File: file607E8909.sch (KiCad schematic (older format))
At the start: 8 parts, among them J1 Conn_01x06_Female, U3 INA4180A1IPWR, U5 254

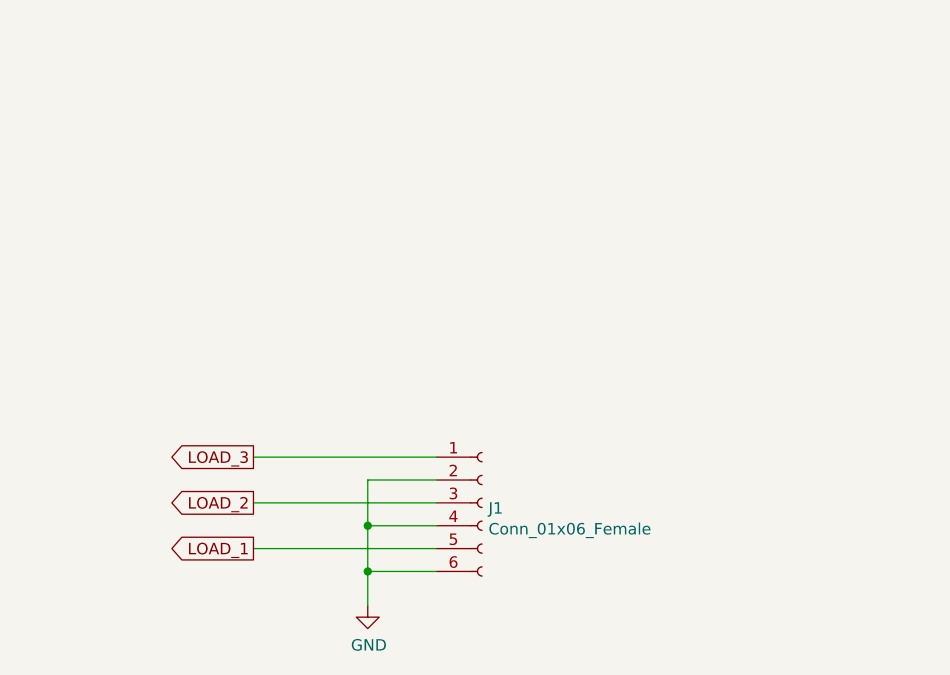
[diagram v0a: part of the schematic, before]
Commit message: incomplete pcb
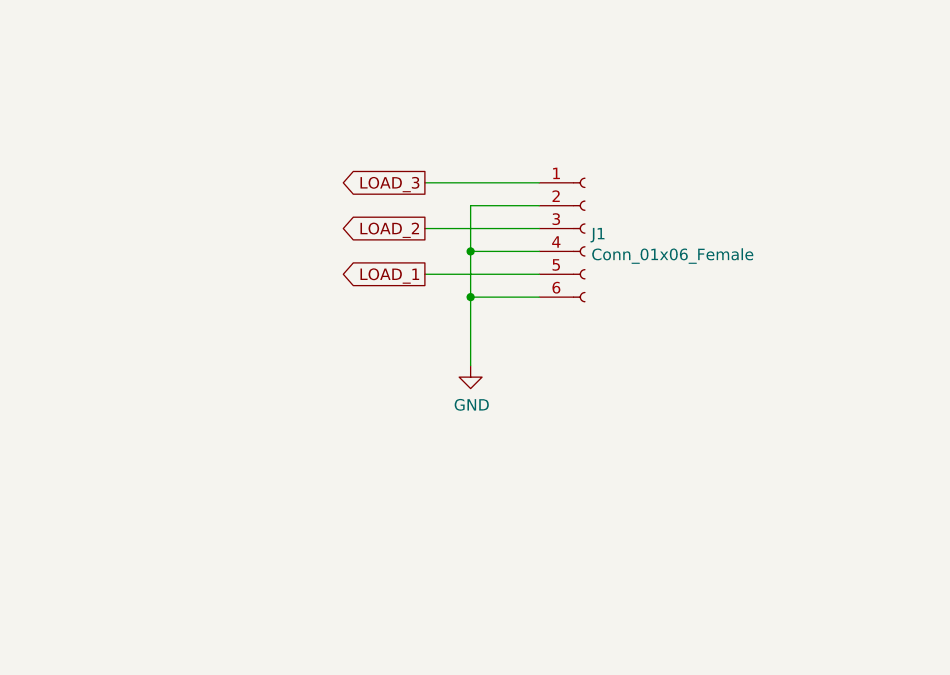
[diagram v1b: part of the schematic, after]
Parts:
- J1: footprint Connector_PinHeader_2.54mm:PinHeader_1x06_P2.54mm_Vertical -> Connector_PinSocket_2.54mm:PinSocket_1x06_P2.54mm_Vertical
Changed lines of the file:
@@
 	9950 2150 10150 2150
 NoConn ~ 10150 2150
+Text GLabel 2400 4150 0    50   Output ~ 0
+LOAD_3
+Wire Wire Line
+	2400 4150 2900 4150
+Wire Wire Line
+	2900 4250 2600 4250
+Wire Wire Line
+	2900 4450 2600 4450
+$Comp
+L power:GND #PWR066
+U 1 1 608EA451
+P 2600 4950
+F 0 "#PWR066" H 2600 4700 50  0001 C CNN
+F 1 "GND" H 2605 4777 50  0000 C CNN
+F 2 "" H 2600 4950 50  0001 C CNN
+F 3 "" H 2600 4950 50  0001 C CNN
+	1    2600 4950
+	1    0    0    -1
+$EndComp
+Text GLabel 2400 4350 0    50   Output ~ 0
+LOAD_2
+Text GLabel 2400 4550 0    50   Output ~ 0
+LOAD_1
+Wire Wire Line
+	2400 4550 2900 4550
 $Comp
 L Connector:Conn_01x06_Female J1
-U 1 1 608A75AE
-P 2650 5550
-F 0 "J1" H 2678 5526 50  0000 L CNN
-F 1 "Conn_01x06_Female" H 2678 5435 50  0000 L CNN
-F 2 "Connector_PinHeader_2.54mm:PinHeader_1x06_P2.54mm_Vertical" H 2650 5550 50  0001 C CNN
-F 3 "~" H 2650 5550 50  0001 C CNN
-	1    2650 5550
-	1    0    0    -1
-$EndComp
-$Comp
-L power:GND #PWR029
-U 1 1 608A8BC9
-P 2150 6000
-F 0 "#PWR029" H 2150 5750 50  0001 C CNN
-F 1 "GND" H 2155 5827 50  0000 C CNN
-F 2 "" H 2150 6000 50  0001 C CNN
-F 3 "" H 2150 6000 50  0001 C CNN
-	1    2150 6000
+U 1 1 6091EFB8
+P 3100 4350
+F 0 "J1" H 3128 4326 50  0000 L CNN
+F 1 "Conn_01x06_Female" H 3128 4235 50  0000 L CNN
+F 2 "Connector_PinSocket_2.54mm:PinSocket_1x06_P2.54mm_Vertical" H 3100 4350 50  0001 C CNN
+F 3 "~" H 3100 4350 50  0001 C CNN
+	1    3100 4350
 	1    0    0    -1
 $EndComp
 Wire Wire Line
-	2150 6000 2150 5850
+	2400 4350 2900 4350
 Wire Wire Line
-	2150 5850 2450 5850
+	2600 4250 2600 4450
 Wire Wire Line
-	2150 5850 2150 5650
+	2900 4650 2600 4650
 Wire Wire Line
-	2150 5650 2450 5650
-Connection ~ 2150 5850
+	2600 4650 2600 4950
 Wire Wire Line
-	2150 5650 2150 5450
-Wire Wire Line
-	2150 5450 2450 5450
-Connection ~ 2150 5650
-Text GLabel 1650 5750 0    50   Output ~ 0
-LOAD_1
-Text GLabel 1650 5550 0    50   Output ~ 0
-LOAD_2
-Text GLabel 1650 5350 0    50   Output ~ 0
-LOAD_3
-Wire Wire Line
-	1650 5350 2450 5350
-Wire Wire Line
-	2450 5550 1650 5550
-Wire Wire Line
-	1650 5750 2450 5750
+	2600 4650 2600 4450
+Connection ~ 2600 4650
+Connection ~ 2600 4450
 $EndSCHEMATC
